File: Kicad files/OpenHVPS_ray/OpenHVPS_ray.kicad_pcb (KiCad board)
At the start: 2 copper layers, 43.4 x 20.6 mm, 70 parts, among them J2 Conn_01x03_Male, Q1 FQT7N10, Q2 BC846A, Q3 MMDT3906, U1 MAX6008AEUR+T, U2 74HC14, U3 MAX4162, U4 CD14538BM

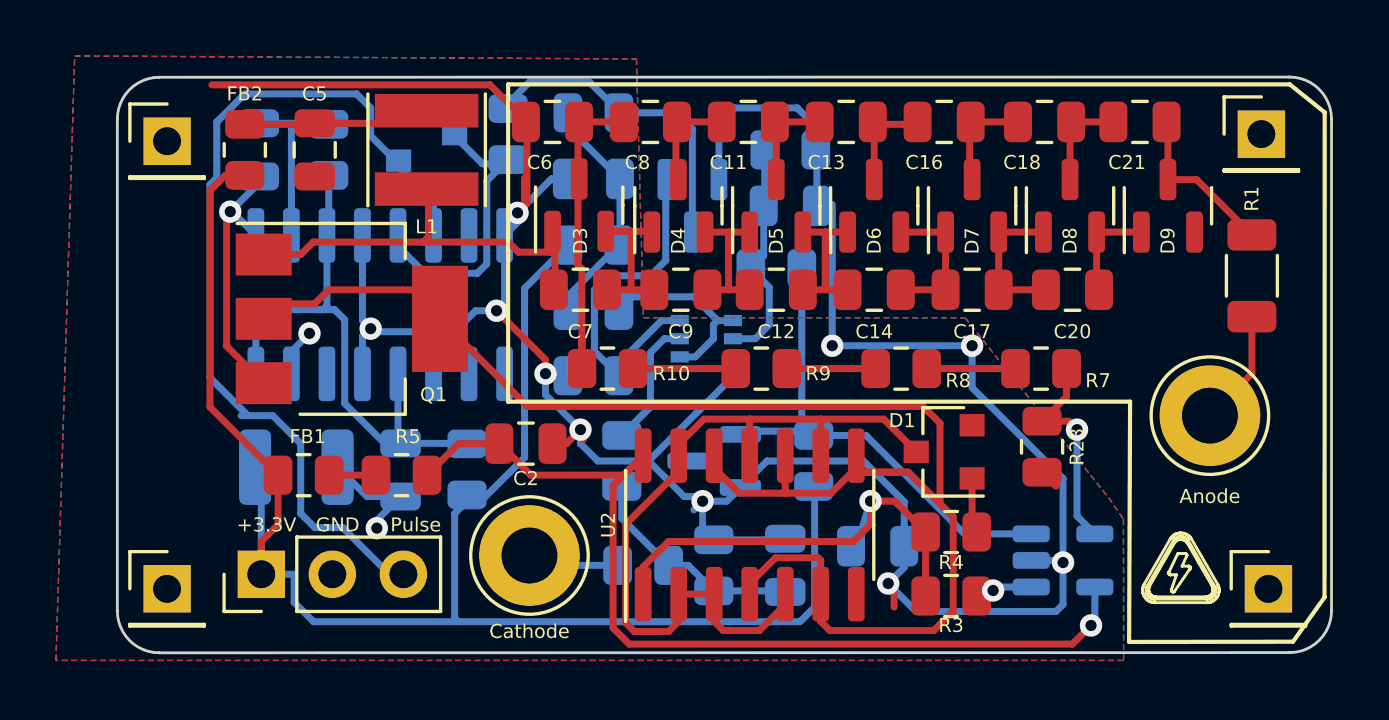
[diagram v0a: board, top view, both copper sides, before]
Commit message: Added Ray version
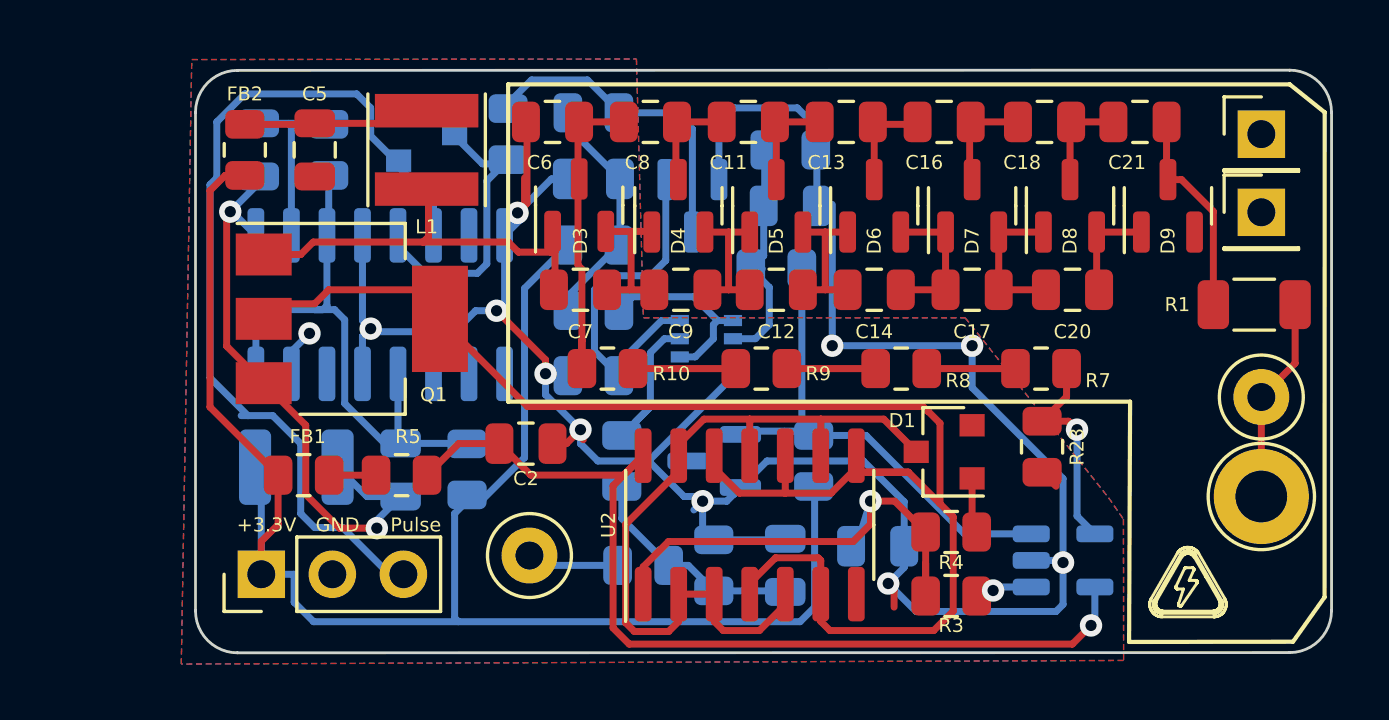
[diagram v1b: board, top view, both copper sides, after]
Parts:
- removed the REF** at (164.6, 75.7)
- removed the REF** at (125.2, 75.7)
- removed the REF** at (125.2, 59.7)
- added ?: LOGO, Symbol:QR_code_SafePulse, F.Cu at (157.2, 66.3)
- added H2: Anode, TestPoint:TestPoint_Loop_D2.50mm_Drill1.85mm, F.Cu at (164.3, 72.4)
- added REF**: PinHeader_1x01_P2.54mm_Vertical, Connector_PinHeader_2.54mm:PinHeader_1x01_P2.54mm_Vertical, F.Cu at (164.3, 62.2)
- H1, H2: footprint TestPoint:TestPoint_Loop_D3.80mm_Drill2.0mm -> TestPoint:TestPoint_Loop_D2.50mm_Drill1.0mm
- moved H2 1.95 mm to (164.3, 68.8)
- moved R1 1.04 mm to (164.1, 65.5), turned to 0 degrees
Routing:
- net GND: track 125.2 -> 121.0 mm
- net Net-(H2-Pad1): track 4.16 -> 8.16 mm
- net Net-(C21-Pad2): track 5.94 -> 7.63 mm
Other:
- board size 43.4 x 20.6 mm -> 40.6 x 20.8 mm
